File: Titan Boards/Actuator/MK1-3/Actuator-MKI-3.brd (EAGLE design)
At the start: 101.6 x 50.8 mm, 57 parts, among them U1 DRV8816PWPR, U2 MBRB2060CTT4G, U3 MBRB2060CTT4G, U4 MBRB2060CTT4G, U5 MBRB2060CTT4G, U6 MBRB2060CTT4G, U7 MBRB2060CTT4G

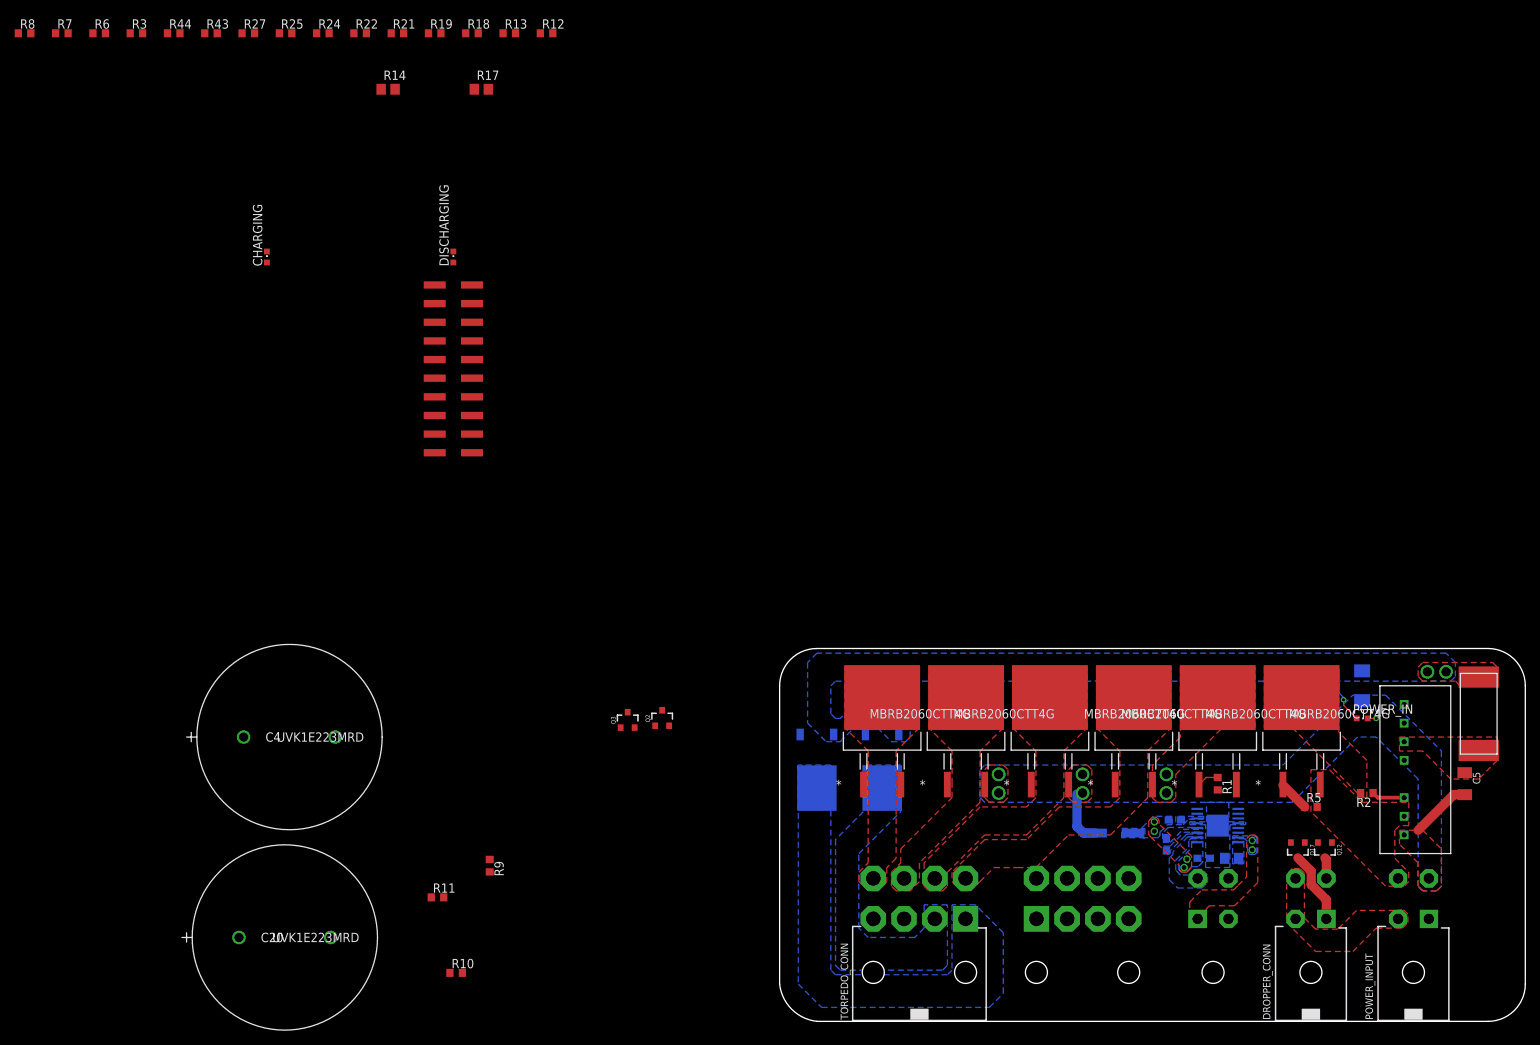
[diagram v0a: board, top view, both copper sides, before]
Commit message: Actuator MK1-3 updates
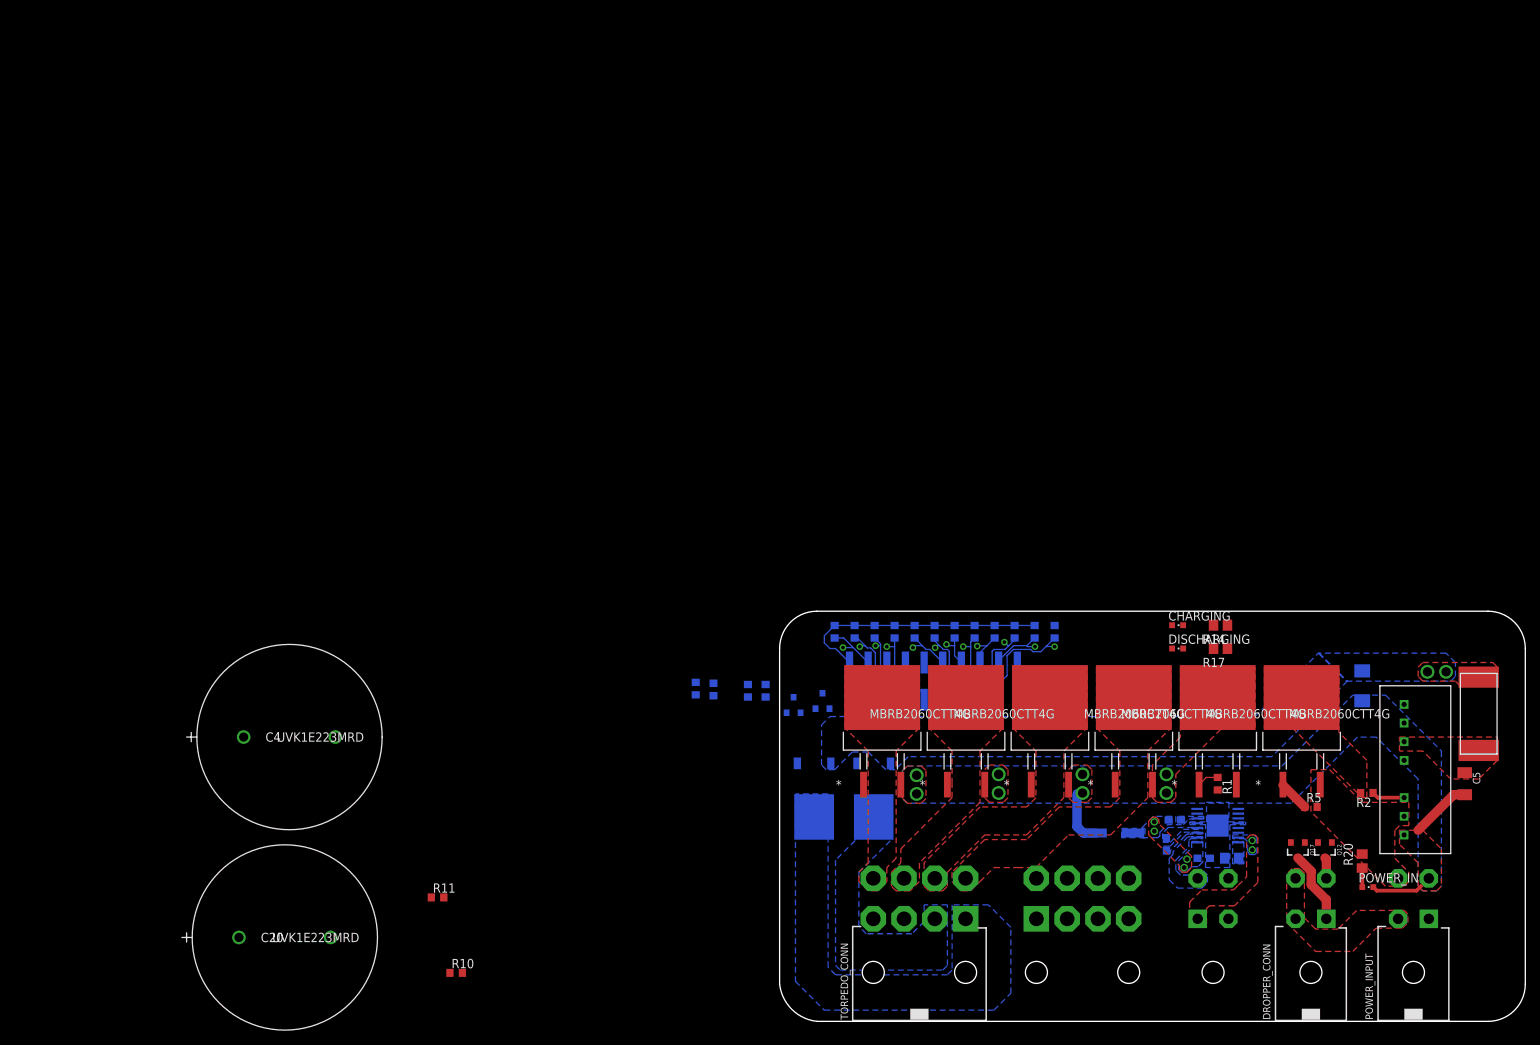
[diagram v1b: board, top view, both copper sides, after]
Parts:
- R10: value 1K -> 10K
- R11: value 150 -> 1.5K
- moved R7 155.6 mm to (34.7, 53.1), flipped to the bottom, turned to 90 degrees
- moved R6 146.7 mm to (29.3, 53.1), flipped to the bottom, turned to 90 degrees
- moved R8 139.4 mm to (10.2, 53.1), flipped to the bottom, turned to 90 degrees
- moved R14 134.9 mm to (60.1, 54.0), turned to 180 degrees
- moved CHARGING 133.8 mm to (54.2, 54.0), turned to 270 degrees
- moved R17 126.3 mm to (60.1, 50.8), turned to 180 degrees
- moved R3 125.3 mm to (7.49, 53.1), flipped to the bottom, turned to 90 degrees
- moved R22 120.8 mm to (32.0, 53.1), flipped to the bottom, turned to 90 degrees
- moved R24 120.6 mm to (26.6, 53.1), flipped to the bottom, turned to 90 degrees
- moved R44 120.5 mm to (-1.91, 45.0), flipped to the bottom, turned to 270 degrees
- moved R25 120.3 mm to (21.1, 53.1), flipped to the bottom, turned to 90 degrees
- moved R27 118.0 mm to (12.9, 53.1), flipped to the bottom, turned to 90 degrees
- moved R19 117.4 mm to (37.5, 53.1), flipped to the bottom, turned to 90 degrees
- moved R43 115.6 mm to (-4.32, 45.0), flipped to the bottom, turned to 90 degrees
- moved DISCHARGING 112.2 mm to (54.2, 50.8), turned to 270 degrees
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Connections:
- new net VPROPI: U$9.P$6, U1.15
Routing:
- net AGND: track 16.9 -> 64.0 mm, vias 7 -> 8
- net TORPEDO2_GATE: track 0.00 -> 15.4 mm, vias 0 -> 1
- net DROPPER2_GATE: track 0.00 -> 12.0 mm, vias 0 -> 1
- net MOTOR_EN: track 0.00 -> 12.0 mm, vias 0 -> 1
- net PWM_DRIVER2: track 0.00 -> 11.3 mm, vias 0 -> 1
- net COIL_4_GATE: track 0.00 -> 10.6 mm, vias 0 -> 1
- net COIL_2_GATE: track 0.00 -> 10.2 mm, vias 0 -> 1
- net ARM_TORPEDO: track 0.00 -> 9.78 mm, vias 0 -> 1
- net COIL_3_GATE: track 0.00 -> 7.59 mm, vias 0 -> 1
- net PWM_DRIVER1: track 0.00 -> 7.35 mm, vias 0 -> 1
- net TORPEDO1_GATE: track 0.00 -> 6.60 mm, vias 0 -> 1
- net COIL_1_GATE: track 0.00 -> 5.47 mm, vias 0 -> 1
- net DROPPER1_GATE: track 0.00 -> 4.91 mm, vias 0 -> 1
- net N$10: track 5.40 -> 2.61 mm, vias 1 -> 0
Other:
- board size 101.6 x 50.8 mm -> 101.6 x 55.9 mm

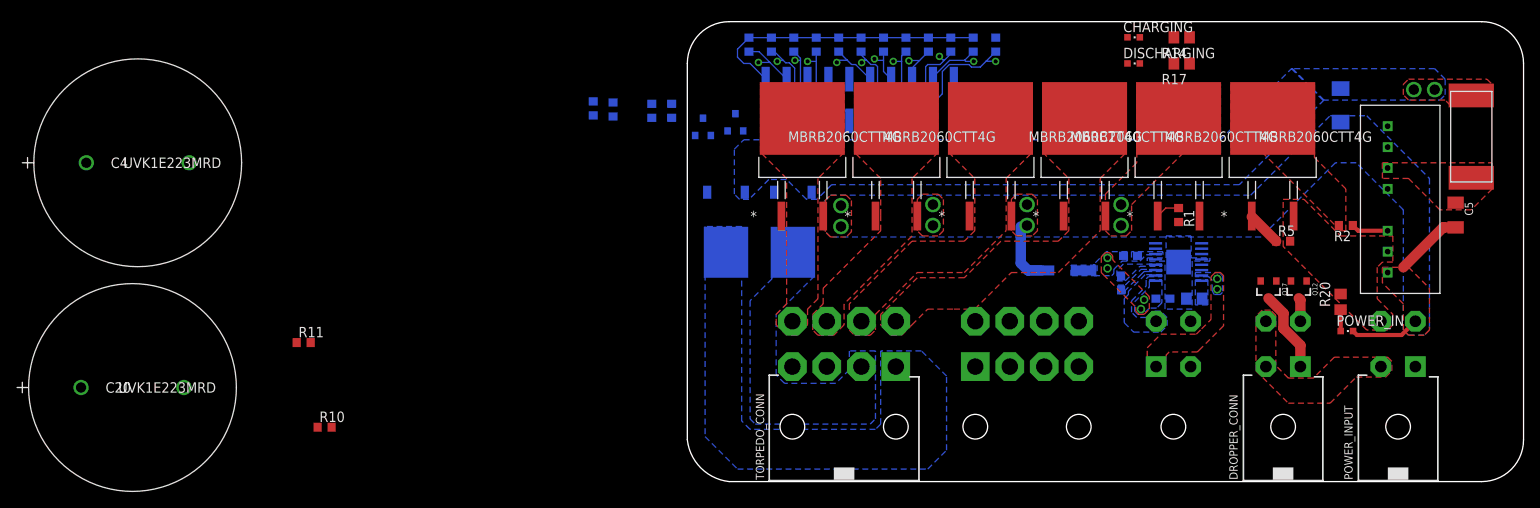
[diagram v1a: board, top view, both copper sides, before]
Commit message: Actuator MKIII updates'
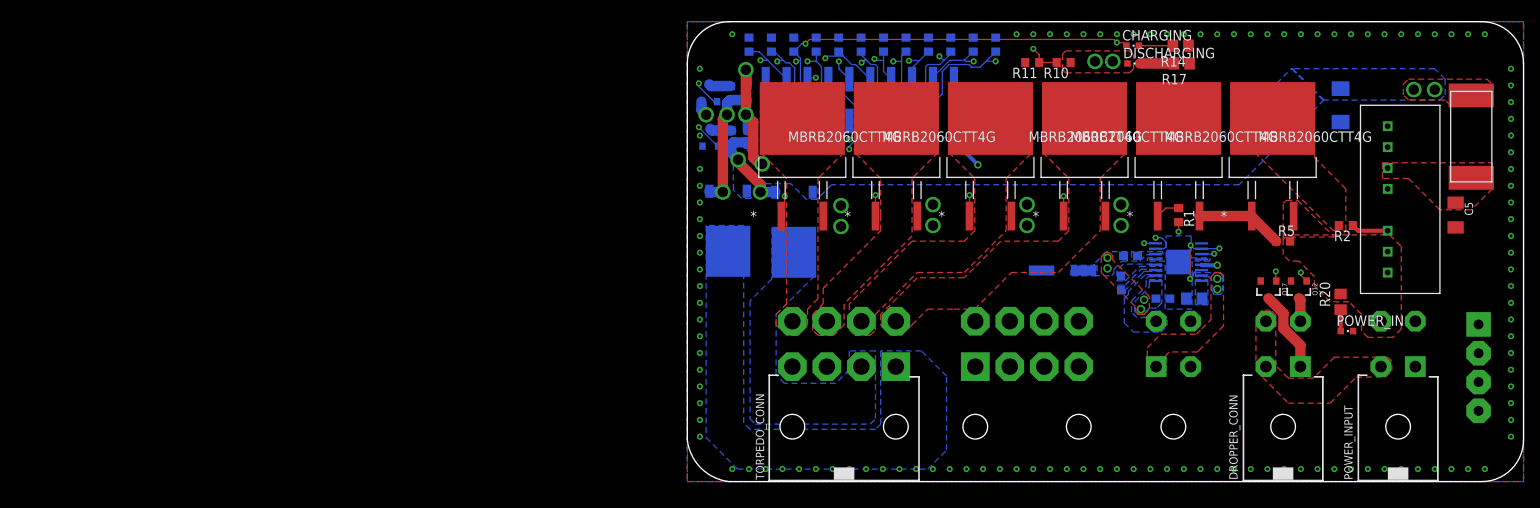
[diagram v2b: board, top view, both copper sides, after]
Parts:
- removed C20, C4: UVK1E223MRD, UVK1E223MRD:CAP_UFW_25X50_NCH
- added U$1: 31059104, 31059104:31059104
- moved R10 100.1 mm to (45.7, 50.9), turned to 180 degrees
- moved R11 94.8 mm to (41.9, 50.9), turned to 180 degrees
- moved R9 19.1 mm to (7.37, 41.8)
- moved R12 14.7 mm to (5.33, 41.8)
- moved R43 11.8 mm to (7.24, 47.2)
- moved R44 7.43 mm to (5.21, 47.2)
- moved Q2 4.77 mm to (2.67, 47.2)
- moved Q3 1.57 mm to (2.79, 41.8)
- moved CHARGING 1.02 mm to (54.1, 53.0)
- moved R14 1.02 mm to (59.9, 53.0)
- moved Q18 0.28 mm to (4.95, 30.5)
- moved Q6 0.13 mm to (13.0, 30.4)
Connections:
- net +24V: now also U$1.P$1, U$1.P$2; no longer C20.1, C4.1
- net AGND: now also U$1.P$3, U$1.P$4; no longer C20.2, C4.2
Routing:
- net +3V3: track 0.00 -> 84.5 mm, vias 0 -> 2
- net MOTOR_EN: track 12.0 -> 87.3 mm, vias 1 -> 4
- net DROPPER1_GATE: track 4.91 -> 77.9 mm, vias 1 -> 2
- net VPROPI: track 0.00 -> 71.7 mm, vias 0 -> 2
- net PWM_DRIVER1: track 7.35 -> 77.8 mm, vias 1 -> 2
- net ARM_TORPEDO: track 9.78 -> 78.3 mm, vias 1 -> 4
- net DROPPER2_GATE: track 12.0 -> 80.4 mm, vias 1 -> 2
- net PWM_DRIVER2: track 11.3 -> 75.2 mm, vias 1 -> 2
- net AGND: track 64.0 -> 7.54 mm, vias 8 -> 127
- net TORPEDO2_GATE: track 15.4 -> 61.4 mm, vias 1 -> 2
- net SDA: track 0.00 -> 44.4 mm, vias 0 -> 1
- net V_DIV: track 0.00 -> 35.1 mm, vias 0 -> 2
- net SCL: track 0.00 -> 32.5 mm, vias 0 -> 1
- net COIL_4_GATE: track 10.6 -> 38.3 mm, vias 1 -> 2
- net COIL_2_GATE: track 10.2 -> 34.6 mm, vias 1 -> 2
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- added copper zone on layer 2, net +12V
- added copper zone on layer 2, net +24V
- added copper zone on layer 15, net AGND
- added copper zone on layer 2, net AGND

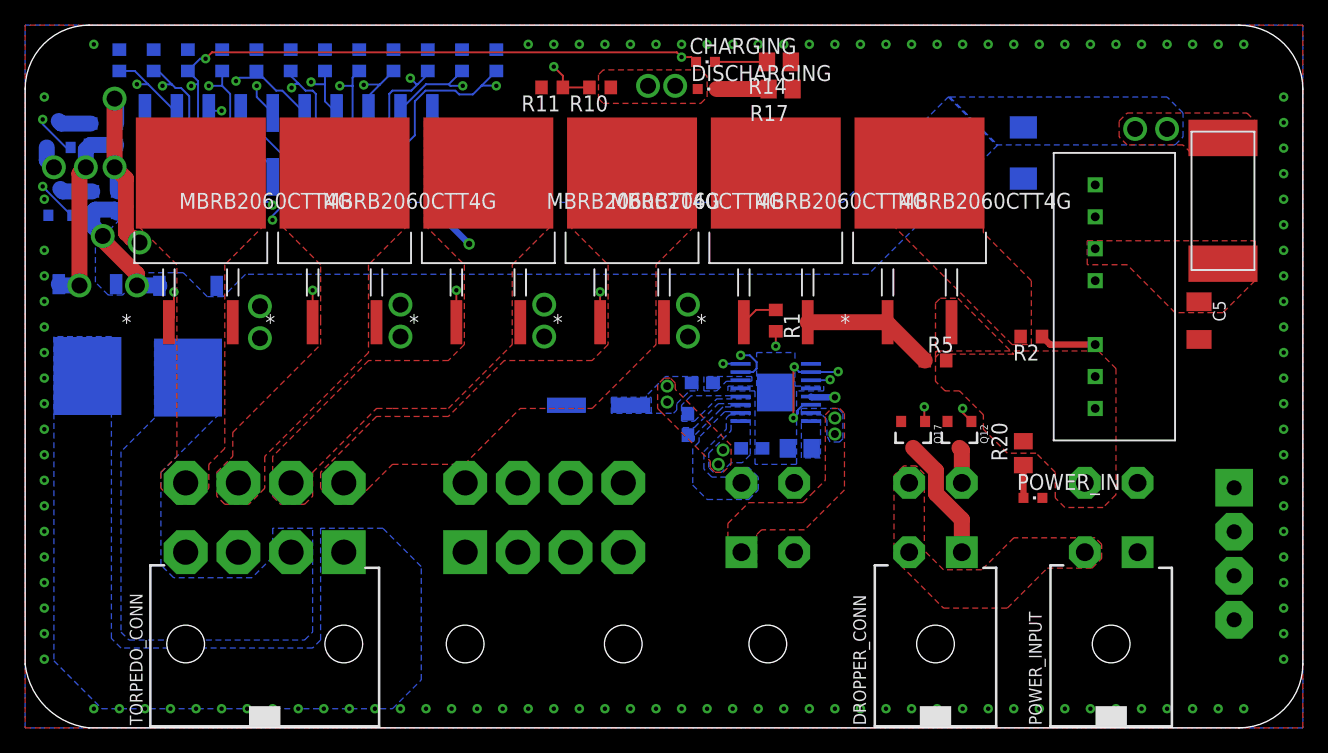
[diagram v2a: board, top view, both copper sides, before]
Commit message: Actuator MK3 for Review
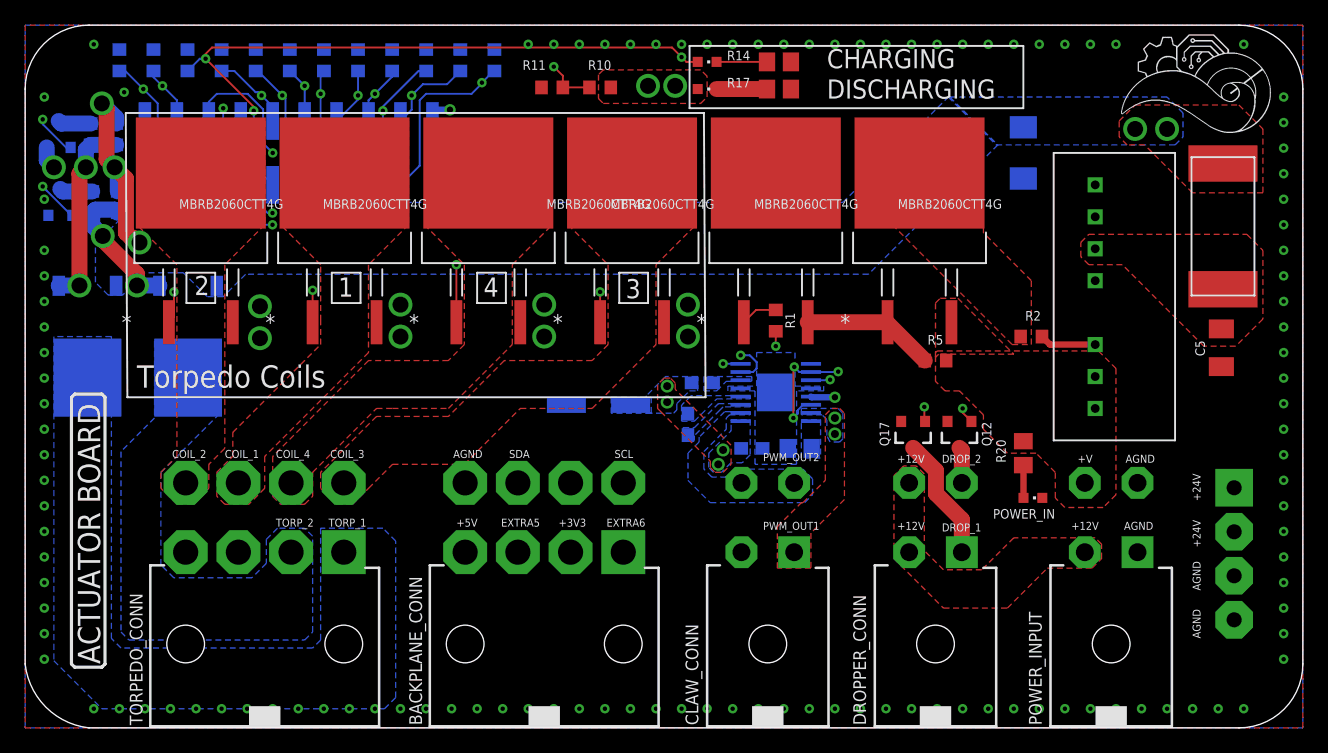
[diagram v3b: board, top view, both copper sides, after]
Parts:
- removed U$9: JTAG-SMD, JTAG-SMD:JTAG-SMD
- added U$2: JTAG-SMD, JTAG-SMD:JTAG-SMD
- moved R18 18.9 mm to (37.3, 53.1)
- moved R7 16.4 mm to (18.3, 53.1)
- moved R21 8.05 mm to (31.9, 53.1)
- moved R6 5.53 mm to (23.8, 53.1)
- moved R19 2.86 mm to (34.6, 53.1)
- moved R22 2.83 mm to (29.2, 53.1)
- moved C5 2.80 mm to (95.1, 30.2)
- moved 120 2.03 mm to (95.2, 39.9)
- moved CHARGING 0.13 mm to (54.2, 53.0)
- moved Q18 0.13 mm to (4.95, 30.4)
- moved R17 0.13 mm to (59.9, 50.8)
- moved R24 0.10 mm to (26.5, 53.1)
- moved R25 0.07 mm to (21.0, 53.1)
- flipped BACKPLANE_CONN to the top
- flipped CLAW_CONN to the top
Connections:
- net +3V3: now also U$2.P$1, U$2.P$11; no longer U$9.P$1, U$9.P$11
- net AGND: now also U$2.P$10, U$2.P$20; no longer U$9.P$10, U$9.P$20
- net ARM_TORPEDO: now also U$2.P$6; no longer U$9.P$18
- net COIL_1_GATE: now also R24.1, U$2.P$14; no longer R6.1, U$9.P$4
- net COIL_2_GATE: now also R6.1, U$2.P$4; no longer R24.1, U$9.P$14
- net COIL_3_GATE: now also R25.1, U$2.P$15; no longer R7.1, U$9.P$5
- net COIL_4_GATE: now also R7.1, U$2.P$5; no longer R25.1, U$9.P$15
- net DROPPER1_GATE: now also U$2.P$3; no longer U$9.P$3
- net DROPPER2_GATE: now also U$2.P$13; no longer U$9.P$13
- net MOTOR_EN: now also U$2.P$16; no longer U$9.P$16
- net PWM_DRIVER1: now also U$2.P$9; no longer U$9.P$9
- net PWM_DRIVER2: now also U$2.P$19; no longer U$9.P$19
- net SCL: now also U$2.P$7; no longer U$9.P$17
- net SDA: now also U$2.P$17; no longer U$9.P$7
- net TORPEDO1_GATE: now also U$2.P$2; no longer U$9.P$2
- net TORPEDO2_GATE: now also U$2.P$12; no longer U$9.P$12
- net VPROPI: now also U$2.P$18; no longer U$9.P$6
- net V_DIV: now also U$2.P$8; no longer U$9.P$8
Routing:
- net TORPEDO1_GATE: track 28.4 -> 54.8 mm
- net MOTOR_EN: track 87.3 -> 71.1 mm
- net TORPEDO2_GATE: track 61.4 -> 46.6 mm
- net VPROPI: track 71.7 -> 59.1 mm
- net PWM_DRIVER2: track 75.2 -> 63.8 mm
- net SCL: track 32.5 -> 42.8 mm
- net COIL_3_GATE: track 30.9 -> 40.4 mm
- net V_DIV: track 35.1 -> 40.9 mm
- net AGND: track 7.54 -> 1.82 mm, vias 127 -> 124
- net DROPPER2_GATE: track 80.4 -> 76.5 mm
- net COIL_4_GATE: track 38.3 -> 34.8 mm
- net +3V3: track 84.5 -> 81.1 mm
- net ARM_TORPEDO: track 78.3 -> 81.5 mm
- net SDA: track 44.4 -> 41.7 mm
- net DROPPER1_GATE: track 77.9 -> 80.3 mm
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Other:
- board text added: "+12V"
- board text added: "+24V"
- board text added: "+3V3"
- board text added: "+5V"
- board text added: "+V"
- board text added: "1"
- board text added: "2"
- board text added: "3"
- board text added: "4"
- board text added: "ACTUATOR BOARD"
- board text added: "AGND"
- board text added: "ARM TORP"
- board text added: "All 10K"
- board text added: "COIL2 GATE"
- board text added: "COIL4 GATE"
- board text added: "COIL_1"
- board text added: "COIL_2"
- board text added: "COIL_3"
- board text added: "COIL_4"
- board text added: "Claw"
- board text added: "DROP1 GATE"
- board text added: "DROP_1"
- board text added: "DROP_2"
- board text added: "EXTRA5"
- board text added: "EXTRA6"
- board text added: "MOTOR EN"
- board text added: "PWM DRV1"
- board text added: "PWM DRV2"
- board text added: "PWM_OUT1"
- board text added: "PWM_OUT2"
- board text added: "SCL"
- board text added: "SDA"
- board text added: "TORP1 GATE"
- board text added: "TORP_1"
- board text added: "TORP_2"
- board text added: "Torpedo Coils"
- board text added: "VDIV"
- board text added: "VPROPI"
